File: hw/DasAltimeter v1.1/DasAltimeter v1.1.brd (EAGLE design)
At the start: 49.1 x 20.6 mm, 57 parts, among them U1 ATSAMD21G-A, U2 MPU-9250, U3 MS5803-14BA, X1 22-23-2041, X2 22-23-2041, Y1 32.768kHx

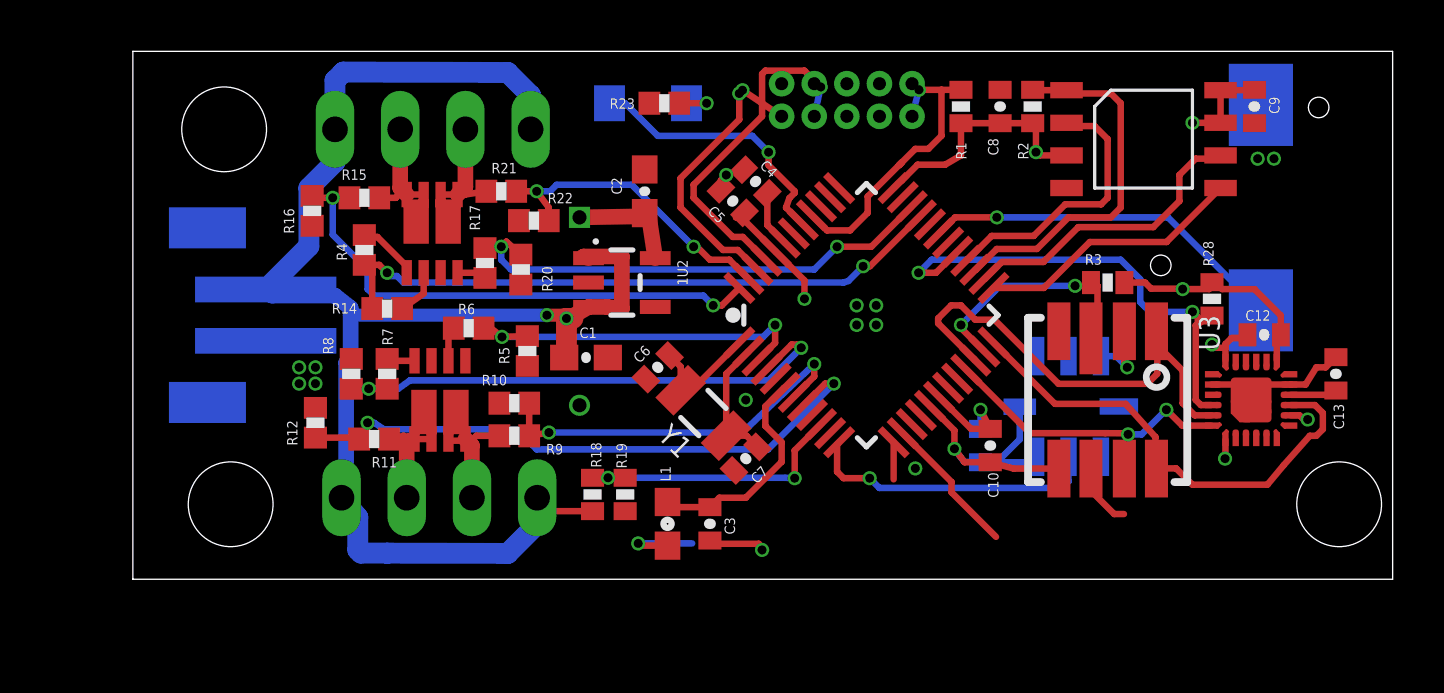
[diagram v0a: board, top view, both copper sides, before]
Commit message: dasaltimeter 1.1 board work
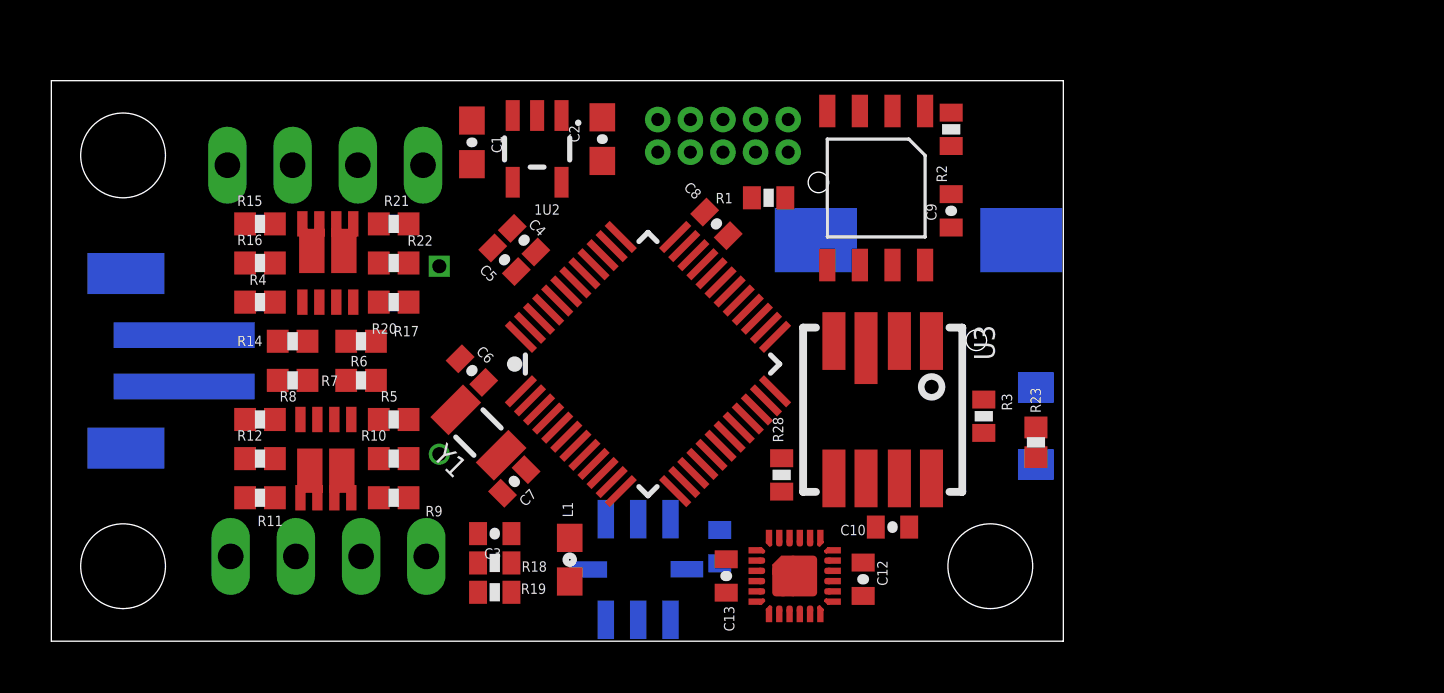
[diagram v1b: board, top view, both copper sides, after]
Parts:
- moved C13 25.0 mm to (26.3, 2.54)
- moved D2 19.7 mm to (38.4, 8.38), turned to 270 degrees
- moved R23 19.6 mm to (38.4, 7.75), turned to 90 degrees
- moved U2 19.1 mm to (29.0, 2.54), turned to 0 degrees
- moved C12 18.3 mm to (31.6, 2.41), turned to 90 degrees
- moved R28 18.1 mm to (28.4, 6.48)
- moved U$7 17.9 mm to (22.9, 2.79), turned to 90 degrees
- moved STANDOFF3 13.8 mm to (36.6, 2.92)
- moved SG1 13.4 mm to (33.8, 15.6), turned to 180 degrees
- moved C9 12.5 mm to (35.1, 16.8), turned to 90 degrees
- moved C8 12.0 mm to (25.9, 16.3), turned to 315 degrees
- moved MEM 11.1 mm to (31.5, 17.7), turned to 270 degrees
- moved C16 10.9 mm to (26.0, 3.68), turned to 270 degrees
- moved C1 9.49 mm to (16.4, 19.4), turned to 270 degrees
- moved C4 9.30 mm to (18.4, 15.6)
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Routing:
- net RAW: track 59.1 -> 0.00 mm, vias 2 -> 0
- net 3.3V: track 59.0 -> 0.00 mm, vias 8 -> 0
- net FIRE_A: track 24.8 -> 0.00 mm, vias 2 -> 0
- net SENSE_D: track 23.7 -> 0.00 mm, vias 2 -> 0
- net GND: track 22.7 -> 0.00 mm, vias 17 -> 0
- net SENSE_A: track 20.8 -> 0.00 mm, vias 2 -> 0
- net FIRE_D: track 20.7 -> 0.00 mm, vias 2 -> 0
- net FIRE_B: track 19.4 -> 0.00 mm, vias 2 -> 0
- net CS_IMU: track 19.0 -> 0.00 mm, vias 2 -> 0
- net SPI1_MISO: track 18.9 -> 0.00 mm
- net SPI1_SCK: track 18.1 -> 0.00 mm
- net SENSE_C: track 15.1 -> 0.00 mm, vias 2 -> 0
- net FIRE_C: track 14.4 -> 0.00 mm, vias 2 -> 0
- net CS_MEM: track 14.4 -> 0.00 mm
- net BUZZER: track 14.3 -> 0.00 mm, vias 1 -> 0
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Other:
- board size 49.1 x 20.6 mm -> 39.4 x 21.8 mm
